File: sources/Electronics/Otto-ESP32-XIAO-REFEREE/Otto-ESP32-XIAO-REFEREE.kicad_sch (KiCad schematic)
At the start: 22 parts, among them J1 Industrial Sensor, J12 OLED 0,91" - I2C (SKU21796), J7 Ultrasonic sensor, J8 Barrel_Jack_Switch, SW1 SW_SPDT, SW4 CherryMX, SW5 CherryMX, SW6 CherryMX, U1 MOUDLE-SEEEDUINO-XIAO-ESP32C3, U2 R-78E5.0-1.0

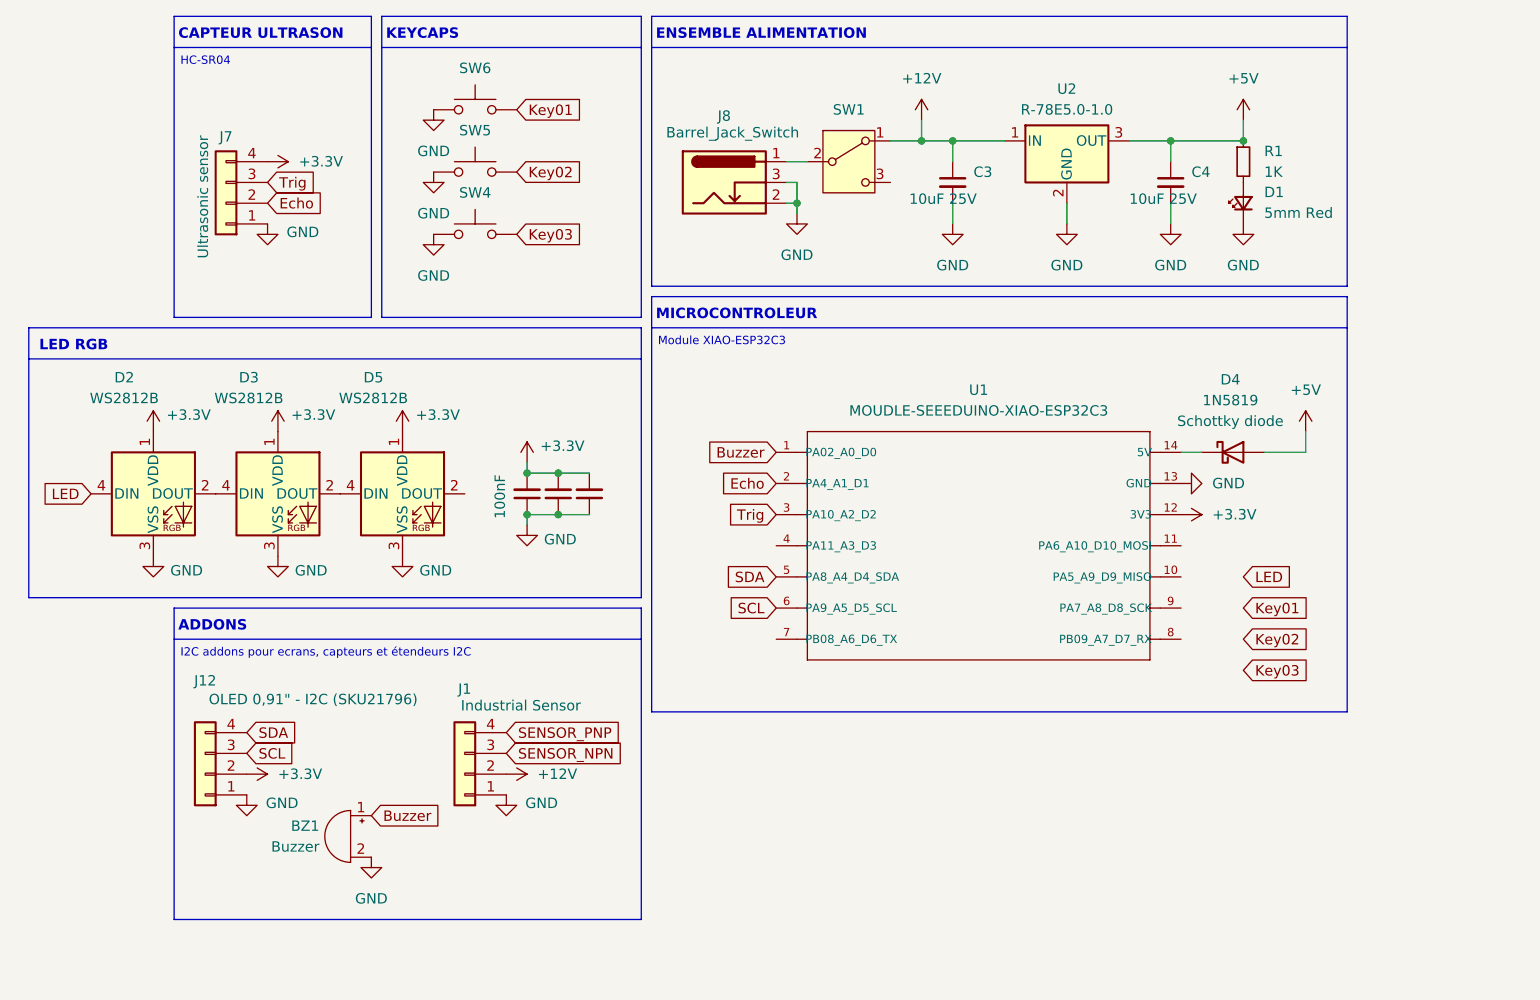
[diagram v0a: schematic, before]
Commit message: update Schematics
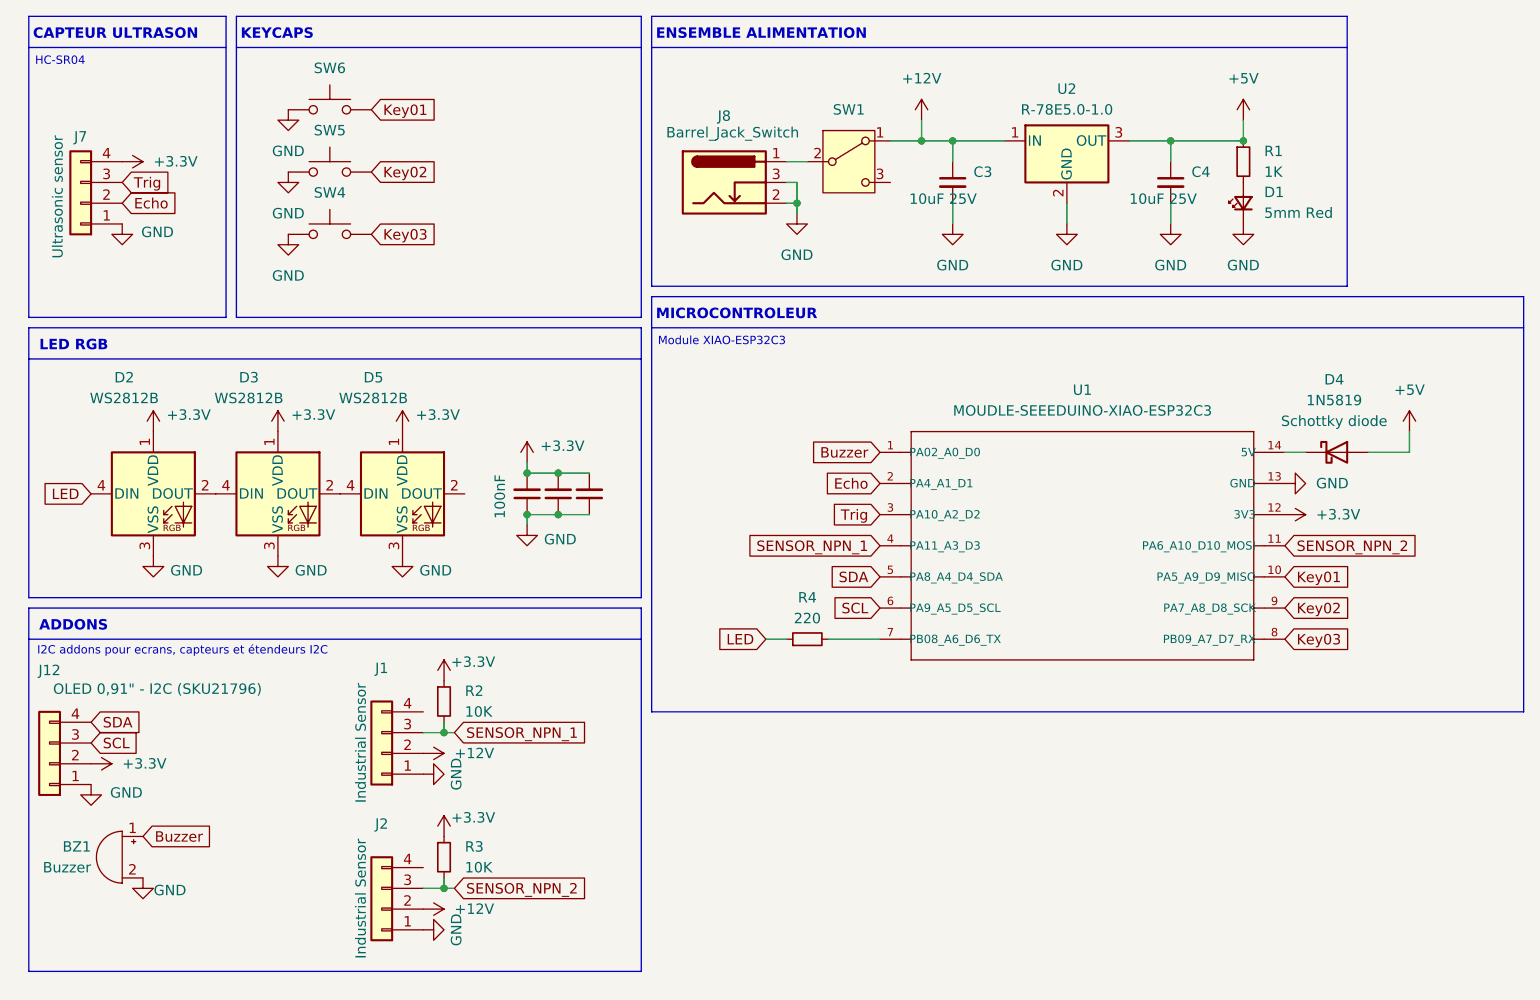
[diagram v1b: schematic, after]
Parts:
- added J2: Industrial Sensor, Connector_Molex:Molex_KK-254_AE-6410-04A_1x04_P2.54mm_Vertical, symbol Connector_Generic:Conn_01x04
- added R2, R3: 10K, Resistor_SMD:R_1206_3216Metric_Pad1.30x1.75mm_HandSolder, symbol Device:R_Small
- added R4: 220, Resistor_SMD:R_1206_3216Metric_Pad1.30x1.75mm_HandSolder, symbol Device:R_Small
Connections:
- net SENSOR_NPN is gone; now on net SENSOR_NPN_1: J1.3 (Pin_3)
- net +12V: now also J2.2 (Pin_2)
- net +3.3V: now also R2.1, R3.1
- net GND: now also J2.1 (Pin_1)
- net Key01: now also U1.10 (PA5_A9_D9_MISO)
- net Key02: now also U1.9 (PA7_A8_D8_SCK)
- net Key03: now also U1.8 (PB09_A7_D7_RX)
- net LED: now also R4.1
- net SENSOR_NPN_2: now reaches U1.11 (PA6_A10_D10_MOSI)
- net SENSOR_NPN_2: now also J2.3 (Pin_3), R3.2
- net SENSOR_NPN_1: now reaches U1.4 (PA11_A3_D3)
- net SENSOR_NPN_1: now also R2.2
- net at U1.7 (PB08_A6_D6_TX): now also R4.2
- net SENSOR_PNP: no longer names the net of J1.4 (Pin_4)
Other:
- moved on the sheet: BZ1, D4, J1, J12, J7, SW4, SW5, SW6, U1
